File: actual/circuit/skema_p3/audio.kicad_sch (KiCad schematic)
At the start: 27 parts, among them U4 MAX98357AETE+, U5 AP2112K-3.3

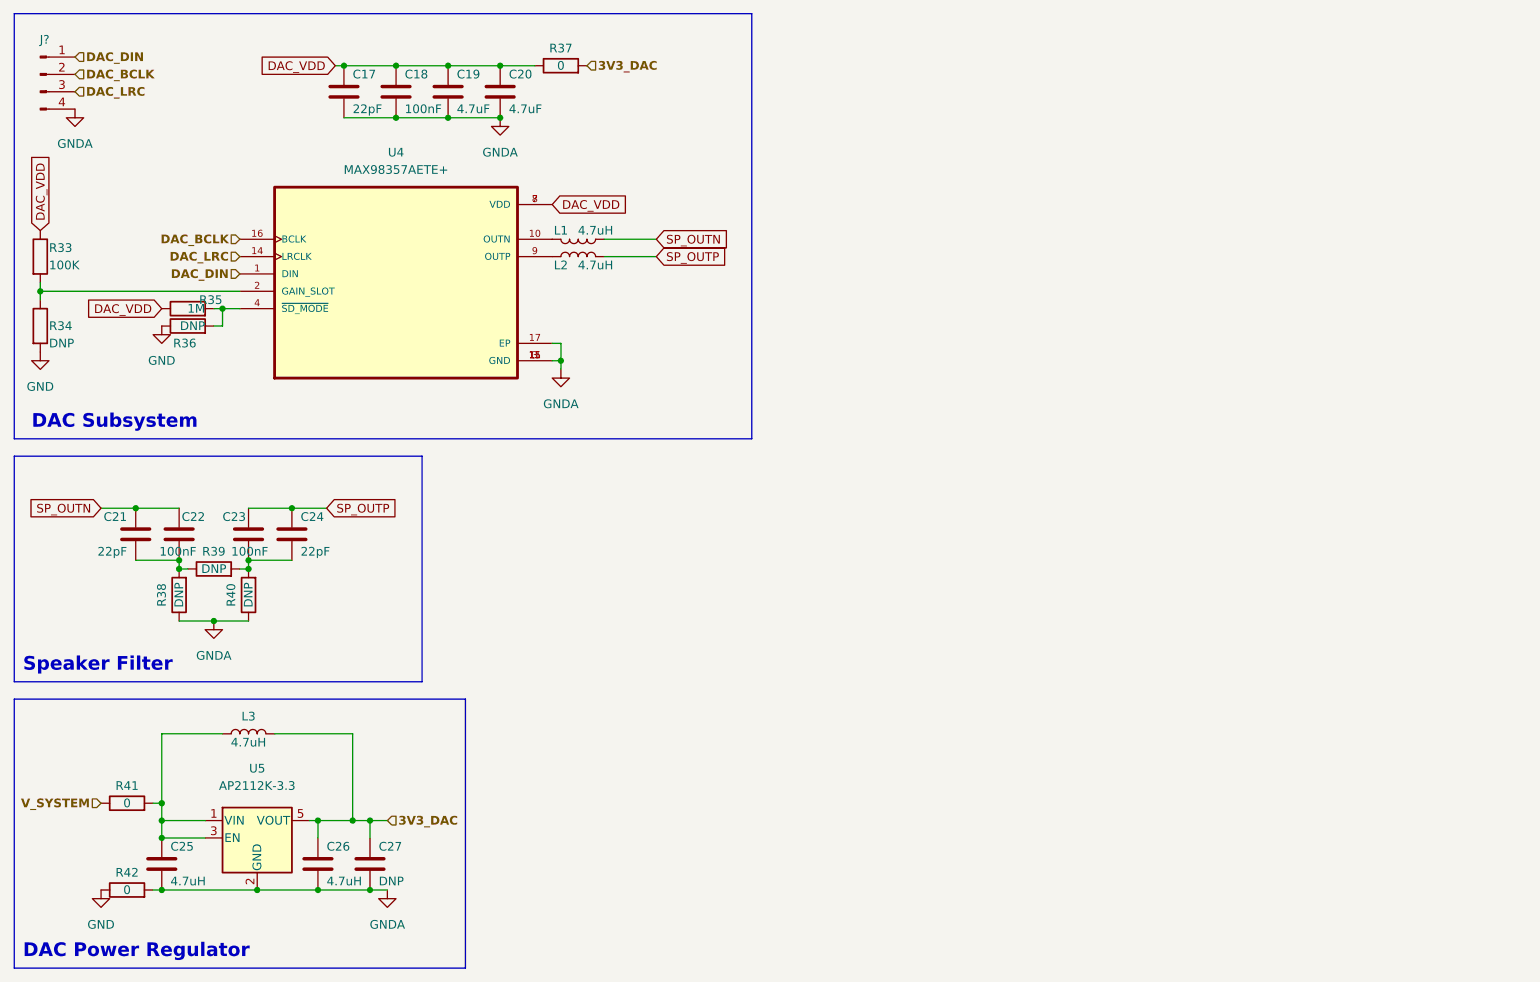
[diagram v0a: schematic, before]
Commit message: P3 in KiCAD
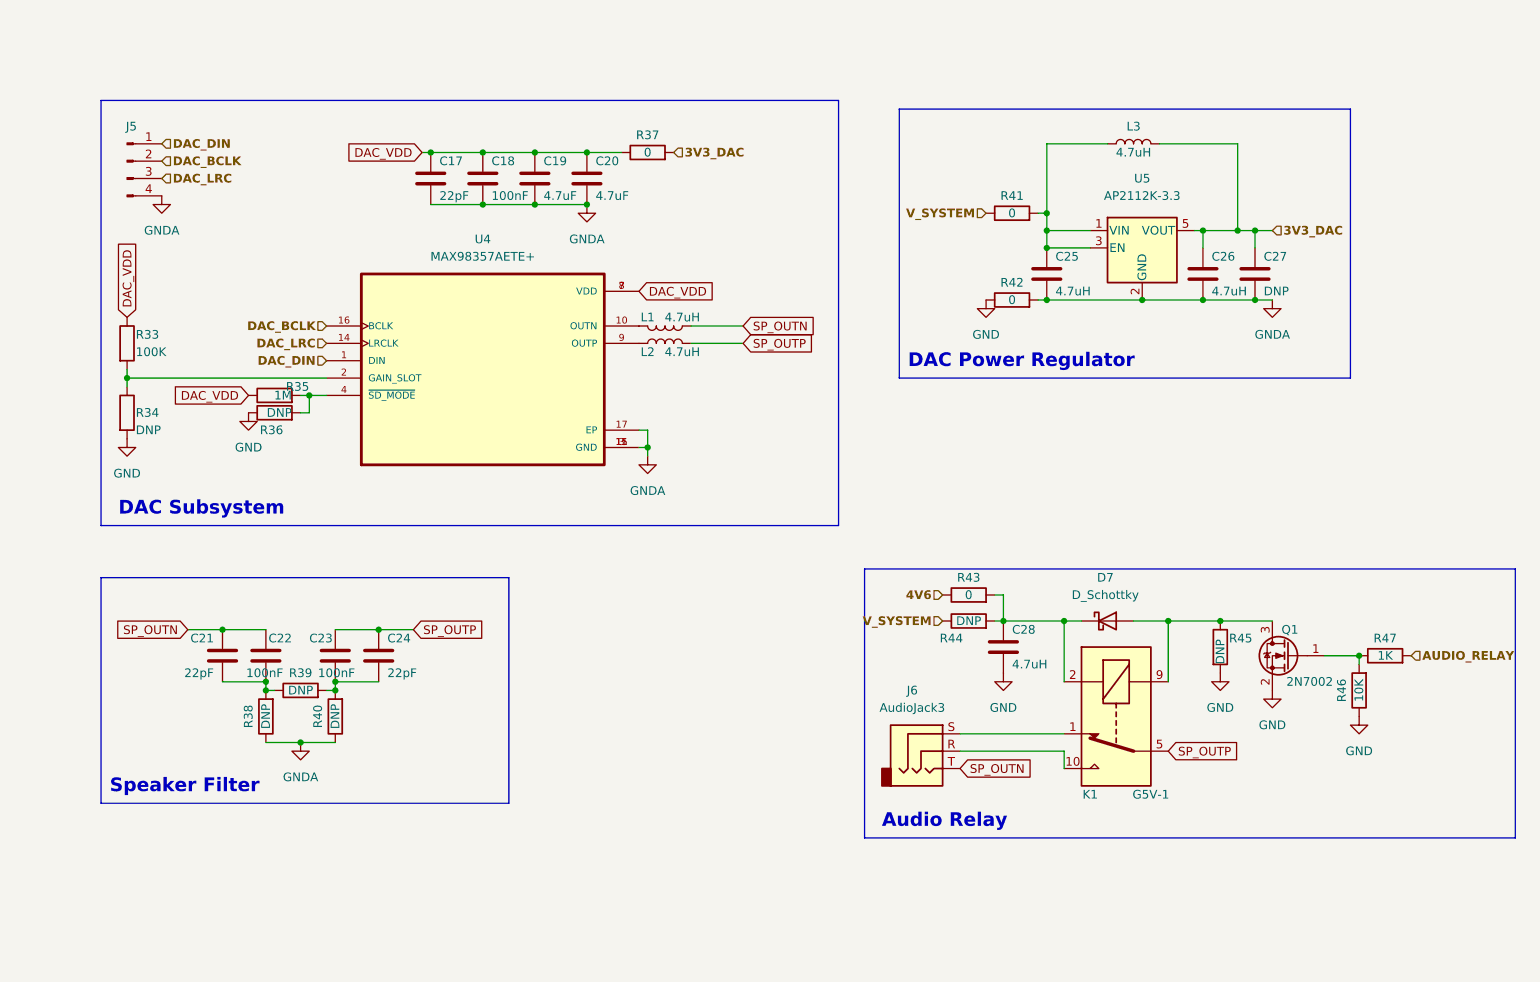
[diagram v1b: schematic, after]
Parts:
- added C28: 4.7uH, symbol Device:C
- added D7: D_Schottky, symbol Device:D_Schottky
- added J6: AudioJack3, symbol Connector:AudioJack3
- added K1: G5V-1, Relay_THT:Relay_SPDT_Omron_G5V-1, symbol Relay:G5V-1
- added Q1: 2N7002, Package_TO_SOT_SMD:SOT-23, symbol Transistor_FET:2N7002
- added R43: 0, symbol Device:R
- added R44, R45: DNP, symbol Device:R
- added R46: 10K, symbol Device:R
- added R47: 1K, symbol Device:R
- gave numbers to parts that had none: 1
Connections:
- net GND: now also C28.2, Q1.2 (S), R45.2, R46.1
- net SP_OUTN: now also J6.T
- net SP_OUTP: now also K1.5, K1.6
- net V_SYSTEM: now also R44.1
- new net: C28.1, D7.1 (K), K1.2, R43.2, R44.2
- new net: D7.2 (A), K1.9, Q1.3 (D), R45.1
- new net: Q1.1 (G), R46.2, R47.1
- new net: J6.R, K1.10
- new net: J6.S, K1.1
- new net 4V6: R43.1
- new net AUDIO_RELAY: R47.2
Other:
- note added: "Audio Relay"
- moved on the sheet: C17, C18, C19, C20, C21, C22, C23, C24, C25, C26, C27, J5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
